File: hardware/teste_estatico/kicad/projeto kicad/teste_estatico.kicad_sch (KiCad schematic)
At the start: 15 parts, among them J1 SDK_GND, J2 SDK_VCC, J3 SDK_MISO, J4 SDK_MOSI, J5 SDK_SCK, J6 SDK_CK

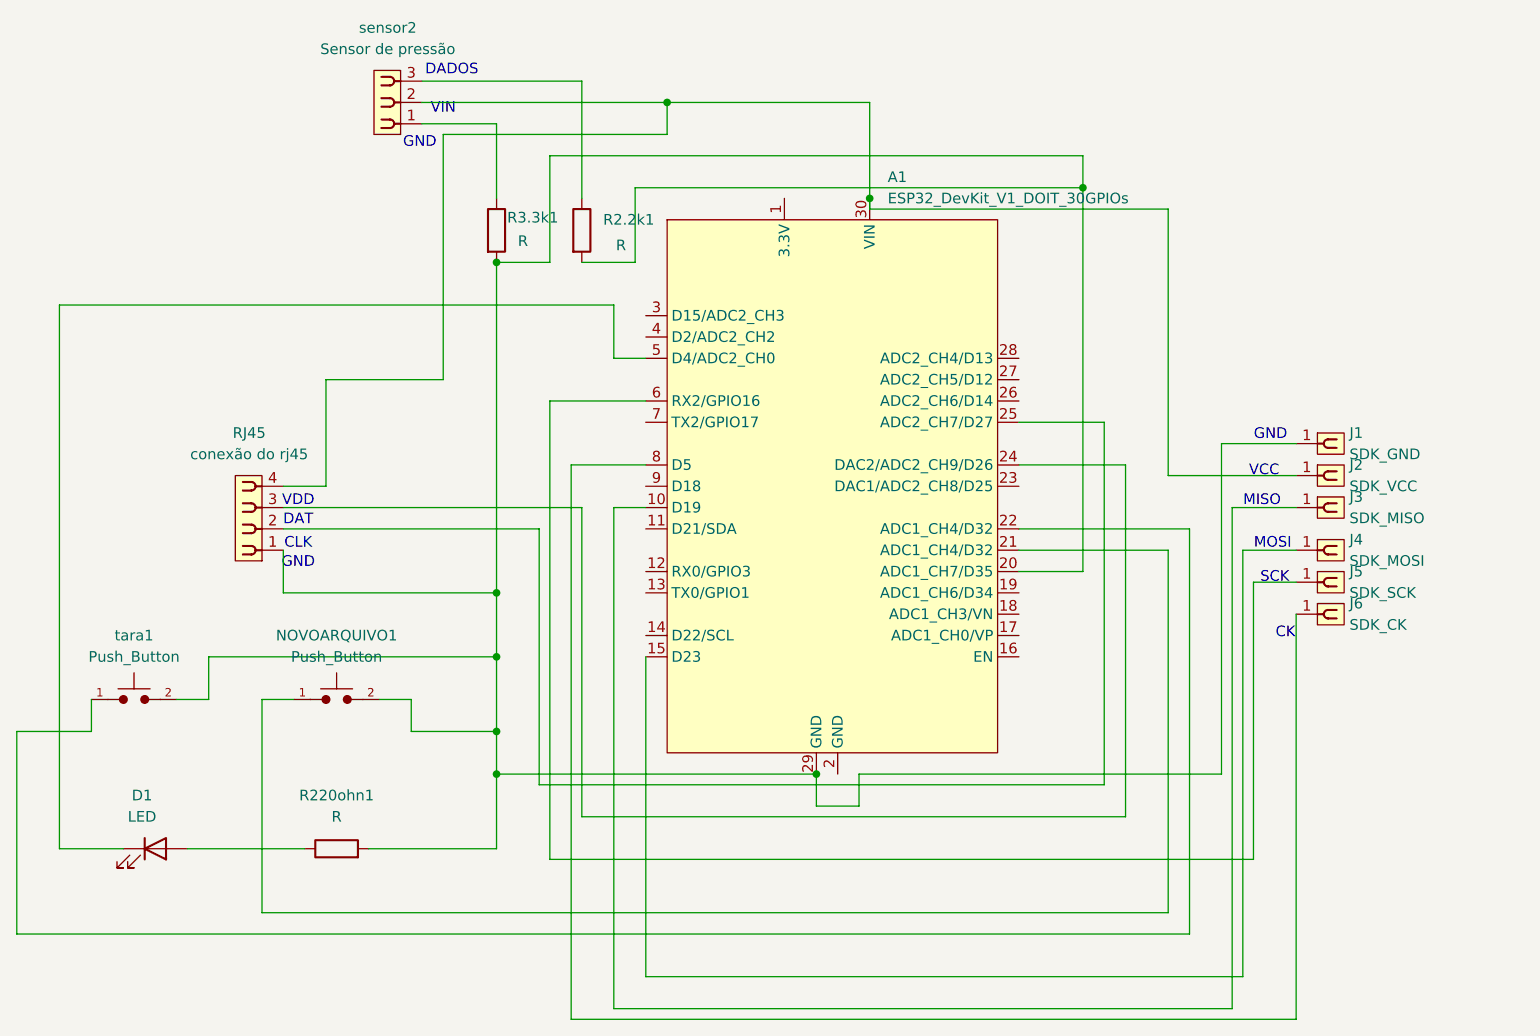
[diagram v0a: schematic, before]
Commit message: chore: atualizando a pcb
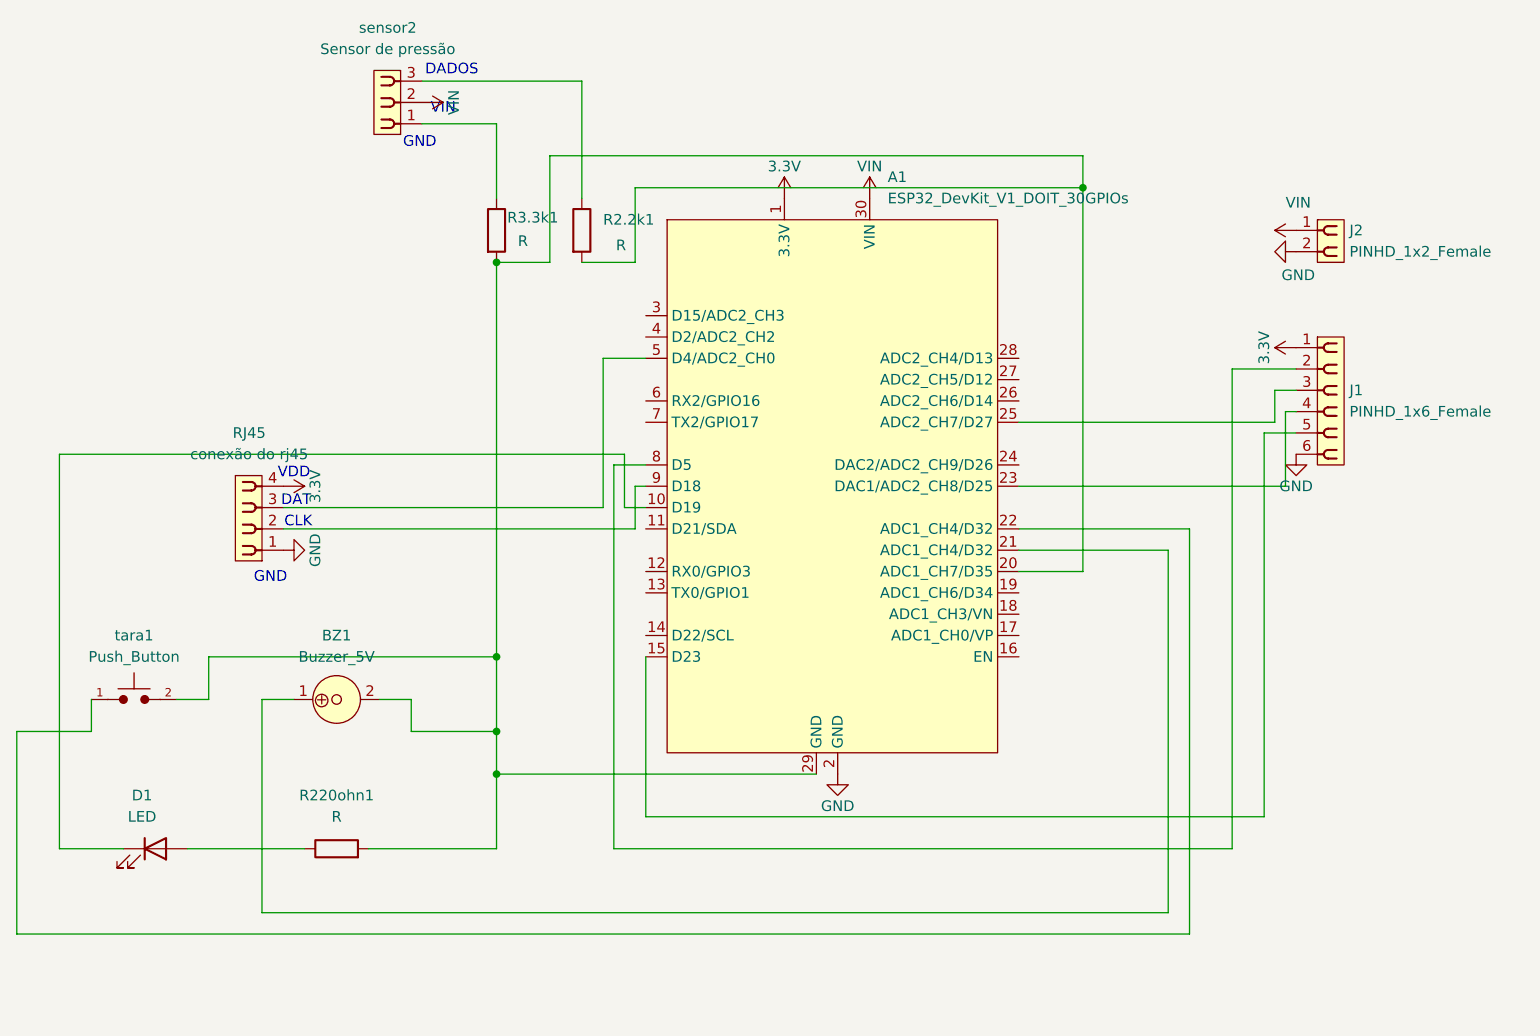
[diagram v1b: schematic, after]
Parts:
- removed J1: SDK_GND, Connector_PinSocket_2.54mm:PinSocket_1x01_P2.54mm_Vertical, symbol PCM_SL_Pin_Headers:PINHD_1x1_Female
- removed J2: SDK_VCC, Connector_PinSocket_2.54mm:PinSocket_1x01_P2.54mm_Vertical, symbol PCM_SL_Pin_Headers:PINHD_1x1_Female
- removed J3: SDK_MISO, Connector_PinSocket_2.54mm:PinSocket_1x01_P2.54mm_Vertical, symbol PCM_SL_Pin_Headers:PINHD_1x1_Female
- removed J4: SDK_MOSI, Connector_PinSocket_2.54mm:PinSocket_1x01_P2.54mm_Vertical, symbol PCM_SL_Pin_Headers:PINHD_1x1_Female
- removed J5: SDK_SCK, Connector_PinSocket_2.54mm:PinSocket_1x01_P2.54mm_Vertical, symbol PCM_SL_Pin_Headers:PINHD_1x1_Female
- removed J6: SDK_CK, Connector_PinSocket_2.54mm:PinSocket_1x01_P2.54mm_Vertical, symbol PCM_SL_Pin_Headers:PINHD_1x1_Female
- removed NOVOARQUIVO1: Push_Button, Button_Switch_THT:SW_PUSH_6mm, symbol PCM_SL_Devices:Push_Button
- added BZ1: Buzzer_5V, Buzzer_Beeper:MagneticBuzzer_ProSignal_ABT-410-RC, symbol PCM_SL_Devices:Buzzer_5V
- added J1: PINHD_1x6_Female, Connector_PinSocket_2.54mm:PinSocket_1x06_P2.54mm_Vertical, symbol PCM_SL_Pin_Headers:PINHD_1x6_Female
- added J2: PINHD_1x2_Female, Connector_PinSocket_2.54mm:PinSocket_1x02_P2.54mm_Vertical, symbol PCM_SL_Pin_Headers:PINHD_1x2_Female
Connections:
- net at A1.21 (ADC1_CH4/D32): now also BZ1.1
- net at A1.20 (ADC1_CH7/D35), A1.29 (GND), R2.2k1.2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: now also BZ1.2; no longer RJ45.1
- net VIN: now reaches A1.30 (VIN), sensor2.2
- net VIN: now also J2.1; no longer RJ45.4
- net 3.3V: now reaches A1.1 (3.3V)
- net 3.3V: now also RJ45.4, J1.1
- net at A1.10 (D19): now also D1.1 (K)
- net at A1.15 (D23): now also J1.5
- net GND: now reaches A1.2 (GND)
- net GND: now also RJ45.1, J1.6, J2.2
- net at A1.23 (DAC1/ADC2_CH8/D25): now also J1.4
- net at A1.24 (DAC2/ADC2_CH9/D26): no longer RJ45.3
- net at A1.25 (ADC2_CH7/D27): now also J1.3; no longer RJ45.2
- net at A1.5 (D4/ADC2_CH0): now also RJ45.3; no longer D1.1 (K)
- net at A1.8 (D5): now also J1.2
- net at A1.9 (D18): now also RJ45.2
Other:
- note removed: "CK"
- note removed: "MISO"
- note removed: "MOSI"
- note removed: "SCK"
- note removed: "VCC"
